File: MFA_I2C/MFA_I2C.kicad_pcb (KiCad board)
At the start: 2 copper layers, 22 parts, among them J1 DIN41612_02x32_AC, J2 Conn_02x04_Odd_Even, SW1 Terminate, SW2 ADR, SW3 INT, U1 74LS00, U2 74LS85, U3 PCF8584, X1 ACO-3MHz-A

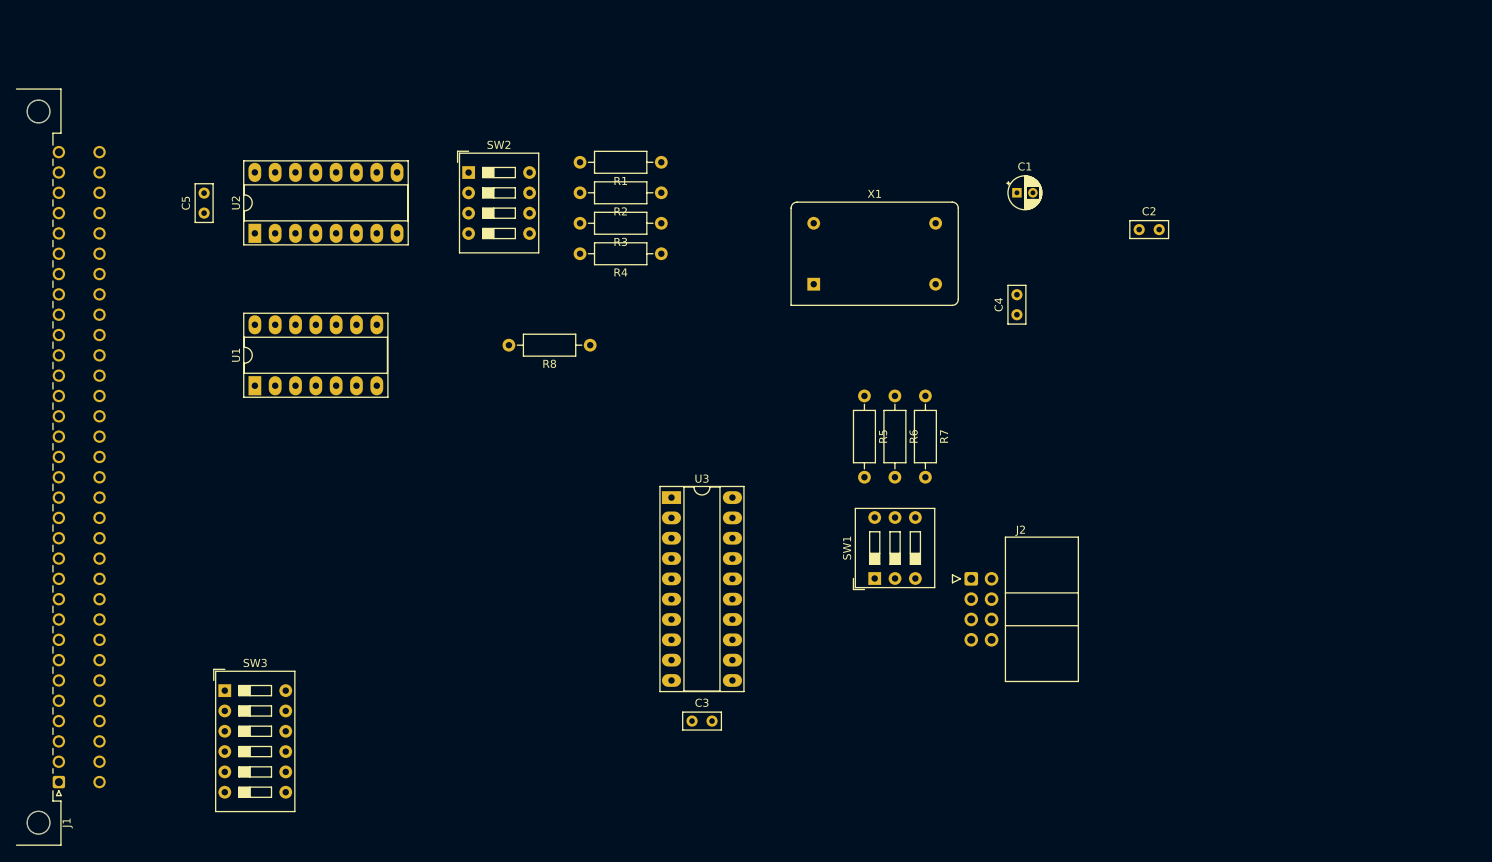
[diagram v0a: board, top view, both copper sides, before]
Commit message: changed
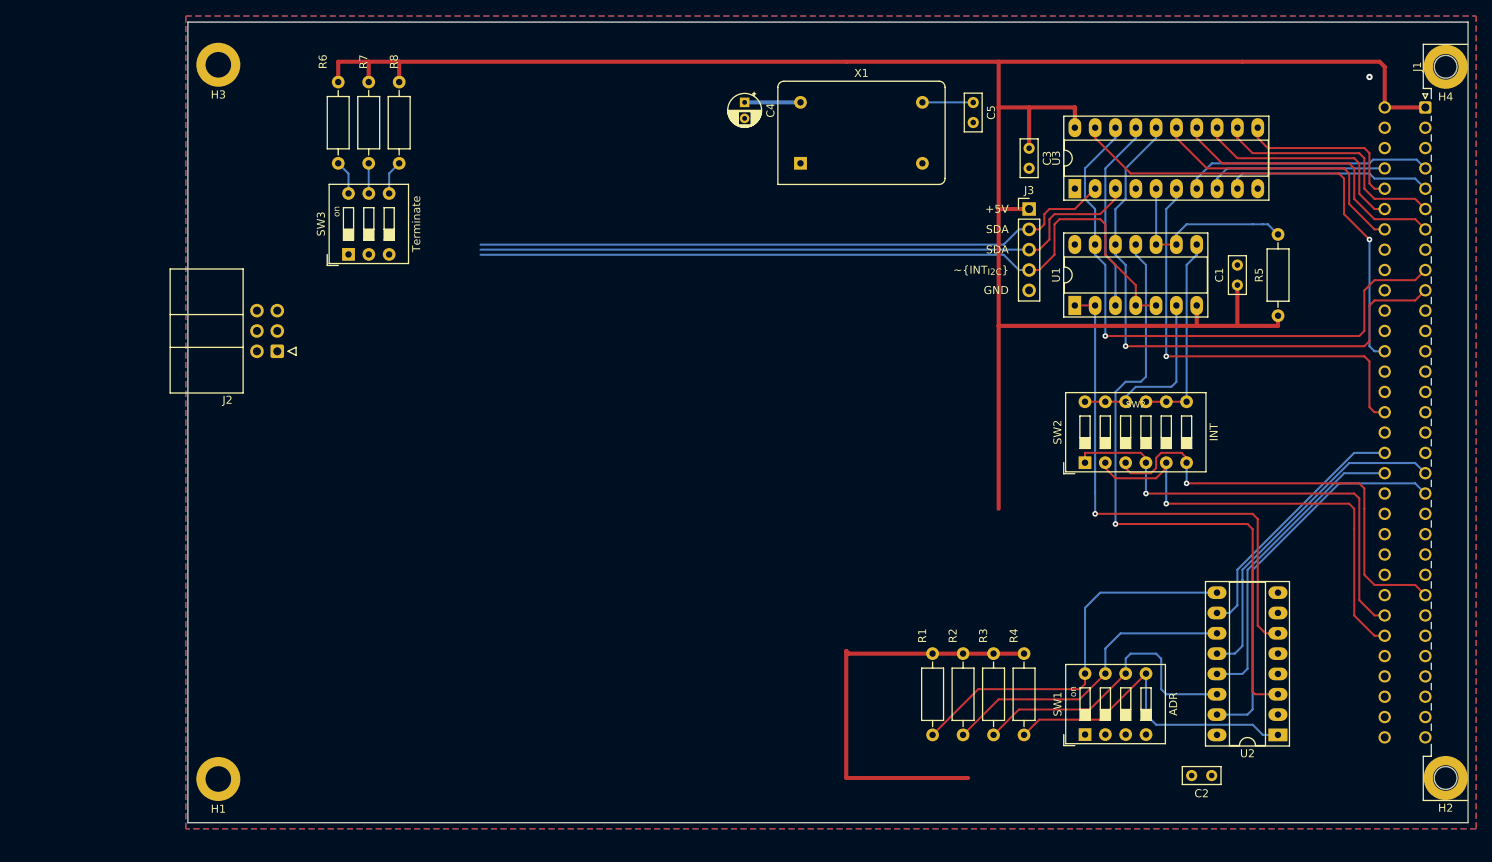
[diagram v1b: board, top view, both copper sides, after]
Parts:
- added H1: MountingHole_Pad, MountingHole:MountingHole_3.2mm_M3_ISO14580_Pad, F.Cu at (78.0, 126.6)
- added H2: MountingHole_Pad, MountingHole:MountingHole_3.2mm_M3_ISO14580_Pad, F.Cu at (231.4, 126.5)
- added H3: MountingHole_Pad, MountingHole:MountingHole_3.2mm_M3_ISO14580_Pad, F.Cu at (78.0, 37.3)
- added H4: MountingHole_Pad, MountingHole:MountingHole_3.2mm_M3_ISO14580_Pad, F.Cu at (231.4, 37.6)
- added J3: Conn_01x05, Connector_PinHeader_2.54mm:PinHeader_1x05_P2.54mm_Vertical, F.Cu at (179.3, 55.4)
- C1: value 10nF -> 0.1uF; footprint Capacitor_THT:CP_Radial_D4.0mm_P2.00mm -> Capacitor_THT:C_Rect_L4.6mm_W2.0mm_P2.50mm_MKS02_FKP02
- C2: value 15pF -> 0.1uF
- C4: value 0.1uF -> 10nF; footprint Capacitor_THT:C_Rect_L4.6mm_W2.0mm_P2.50mm_MKS02_FKP02 -> Capacitor_THT:CP_Radial_D4.0mm_P2.00mm
- C5: value 0.1uF -> 15pF
- J2: value Conn_02x04_Odd_Even -> Conn_02x03_Odd_Even; footprint Connector_IDC:IDC-Header_2x04_P2.54mm_Horizontal -> Connector_IDC:IDC-Header_2x03_P2.54mm_Horizontal
- SW1: value Terminate -> ADR; footprint Button_Switch_THT:SW_DIP_SPSTx03_Slide_9.78x9.8mm_W7.62mm_P2.54mm -> Button_Switch_THT:SW_DIP_SPSTx04_Slide_9.78x12.34mm_W7.62mm_P2.54mm
- SW2: value ADR -> INT; footprint Button_Switch_THT:SW_DIP_SPSTx04_Slide_9.78x12.34mm_W7.62mm_P2.54mm -> Button_Switch_THT:SW_DIP_SPSTx06_Slide_9.78x17.42mm_W7.62mm_P2.54mm
- SW3: value INT -> Terminate; footprint Button_Switch_THT:SW_DIP_SPSTx06_Slide_9.78x17.42mm_W7.62mm_P2.54mm -> Button_Switch_THT:SW_DIP_SPSTx03_Slide_9.78x9.8mm_W7.62mm_P2.54mm
- moved J1 190.5 mm to (228.9, 42.7), turned to -90 degrees
- moved U2 142.4 mm to (210.4, 121.1), turned to 180 degrees
- moved U1 103.0 mm to (185.0, 67.4)
- moved C5 97.1 mm to (172.3, 42.1), turned to -90 degrees
- moved J2 91.3 mm to (85.3, 73.2), turned to 180 degrees
- moved SW2 85.2 mm to (186.3, 87.1), turned to 90 degrees
- moved C3 83.1 mm to (179.3, 47.8), turned to -90 degrees
- moved R6 79.9 mm to (93.0, 39.5)
- moved R7 79.9 mm to (96.8, 39.5)
- moved R1 70.2 mm to (167.3, 110.9), turned to -90 degrees
- moved R2 68.9 mm to (171.1, 110.9), turned to -90 degrees
- moved C2 68.8 mm to (202.1, 126.2), turned to 180 degrees
- moved R3 68.0 mm to (174.9, 110.9), turned to -90 degrees
- moved R4 67.5 mm to (178.7, 110.9), turned to -90 degrees
- moved U3 63.5 mm to (185.0, 52.8), turned to 90 degrees
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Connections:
- C2 pad 1: /CLK_{I2C} -> VCC
- C5 pad 1: VCC -> /CLK_{I2C}
- J2 pad 2: VCC -> /~{INT_{I2C}}
- J2 pad 4: /SCL -> GND
- J2 pad 5: /~{INT_{I2C}} -> /SCL
- J2 pad 6: unconnected-(J2-Pad6) -> GND
- R5 pad 2: Net-(R5-Pad2) -> /~{INT}
- R8 pad 2: /~{INT} -> Net-(R8-Pad2)
- SW1 pad 1: /SDA -> GND
- SW1 pad 2: /SCL -> GND
- SW1 pad 3: /~{INT_{I2C}} -> GND
- SW1 pad 4: Net-(R7-Pad2) -> GND
- SW1 pad 5: Net-(R6-Pad2) -> /B_{7}
- SW1 pad 6: Net-(R5-Pad2) -> /B_{6}
- SW2 pad 1: GND -> /RST_{5.5}
- SW2 pad 2: GND -> /RST_{6.5}
- SW2 pad 3: GND -> /RST_{7.5}
- SW2 pad 4: GND -> /RST_{5.5}
- SW2 pad 5: /B_{7} -> /RST_{6.5}
- SW2 pad 6: /B_{6} -> /RST_{7.5}
- SW2 pad 7: /B_{5} -> /INT
- SW2 pad 8: /B_{4} -> /INT
- SW3 pad 1: /RST_{5.5} -> /SDA
- SW3 pad 2: /RST_{6.5} -> /SCL
- SW3 pad 3: /RST_{7.5} -> /~{INT_{I2C}}
- SW3 pad 4: /RST_{5.5} -> Net-(R8-Pad2)
- SW3 pad 5: /RST_{6.5} -> Net-(R7-Pad2)
- SW3 pad 6: /RST_{7.5} -> Net-(R6-Pad2)
- U1 pad 11: Net-(SW3-Pad7) -> /IOWR
- U1 pad 12: /~{INT_{I2C}} -> /~{IOR}
- U1 pad 13: /~{INT_{I2C}} -> /~{IOW}
- U1 pad 4: /~{IOR} -> /~{INT_{I2C}}
- U1 pad 5: /~{IOW} -> /~{INT_{I2C}}
- U1 pad 6: /IOWR -> /INT_{I2C}
- U1 pad 8: Net-(SW3-Pad10) -> /INT
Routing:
- net VCC: track 0.00 -> 330.0 mm
- net /~{INT_{I2C}}: track 0.00 -> 98.3 mm
- net /SCL: track 0.00 -> 84.8 mm
- net /SDA: track 0.00 -> 80.5 mm
- net /IOWR: track 0.00 -> 79.2 mm, vias 0 -> 1
- net /~{IOW}: track 0.00 -> 75.1 mm, vias 0 -> 1
- net /~{IOR}: track 0.00 -> 72.9 mm, vias 0 -> 1
- net /a=b: track 0.00 -> 65.4 mm, vias 0 -> 1
- net /~{RESOUT}: track 0.00 -> 58.9 mm, vias 0 -> 1
- net /RST_{5.5}: track 0.00 -> 57.2 mm, vias 0 -> 1
- net /RST_{6.5}: track 0.00 -> 57.1 mm, vias 0 -> 1
- net /RST_{7.5}: track 0.00 -> 55.7 mm, vias 0 -> 1
- net /A_{0}: track 0.00 -> 55.0 mm, vias 0 -> 1
- net /A_{7}: track 0.00 -> 48.8 mm
- net /B_{4}: track 0.00 -> 48.5 mm
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- added copper zone on B.Cu, net GND
- added copper zone on F.Cu, net GND
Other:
- board outline added: 160 x 100.1 mm
- board text added: "+5V"
- board text added: "GND"
- board text added: "SDA"
- board text added: "~{INT_{I2C}}"
